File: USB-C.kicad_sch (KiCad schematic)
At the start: 32 parts, among them IC2 TPS2557QDRBTQ1, IC5 TPS2557QDRBTQ1, IC7 TPS2557QDRBTQ1, J10 USB_C_Receptacle, J5 USB_C_Receptacle_USB2.0_16P, J7 USB_C_Receptacle_USB2.0_16P

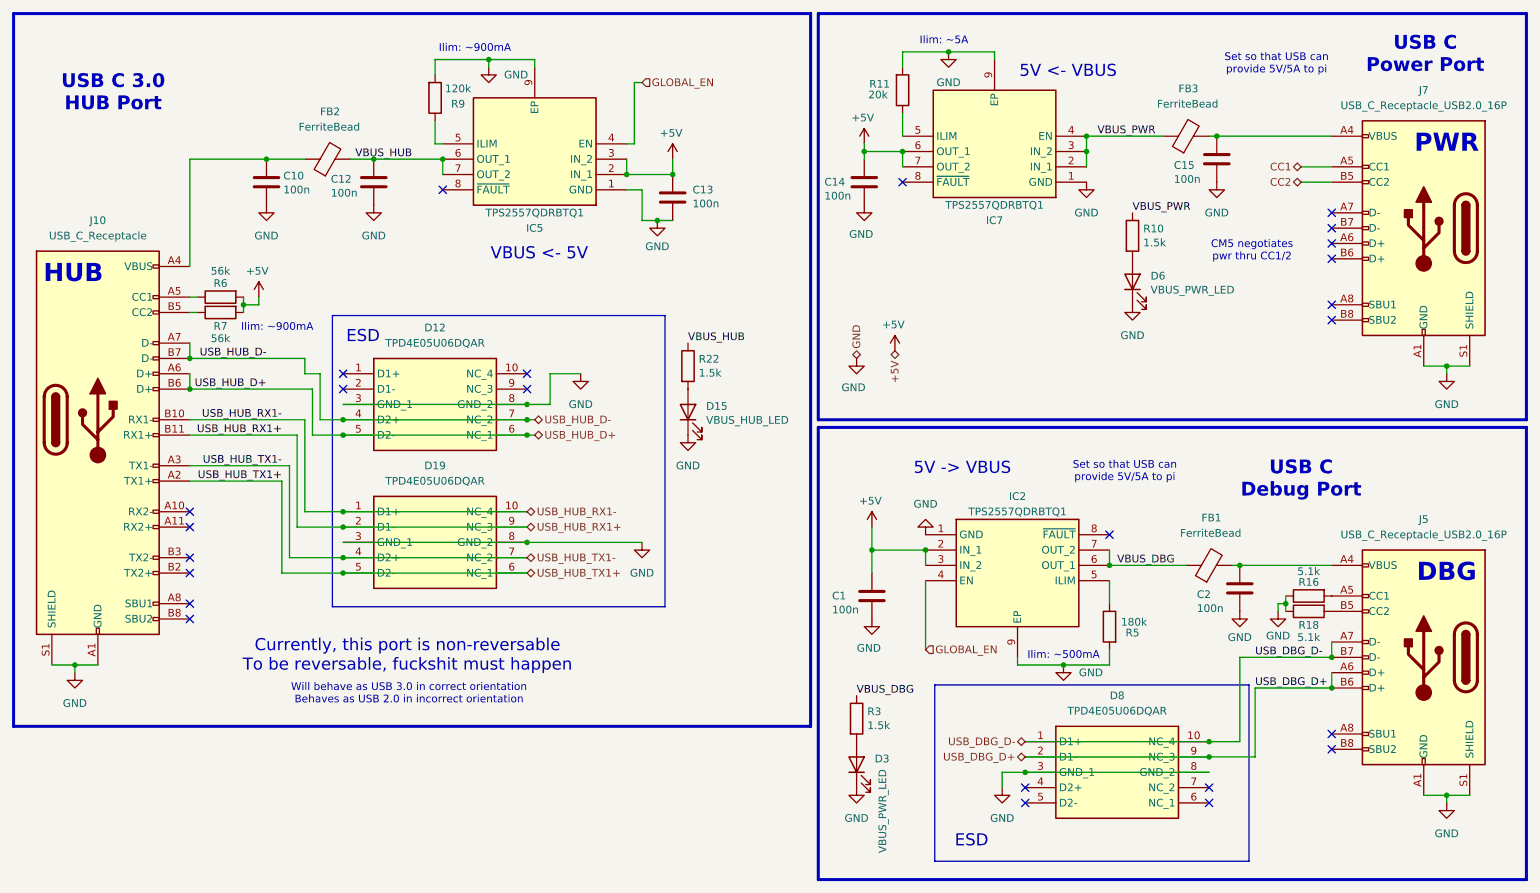
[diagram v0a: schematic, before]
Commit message: wow everything could not be worse
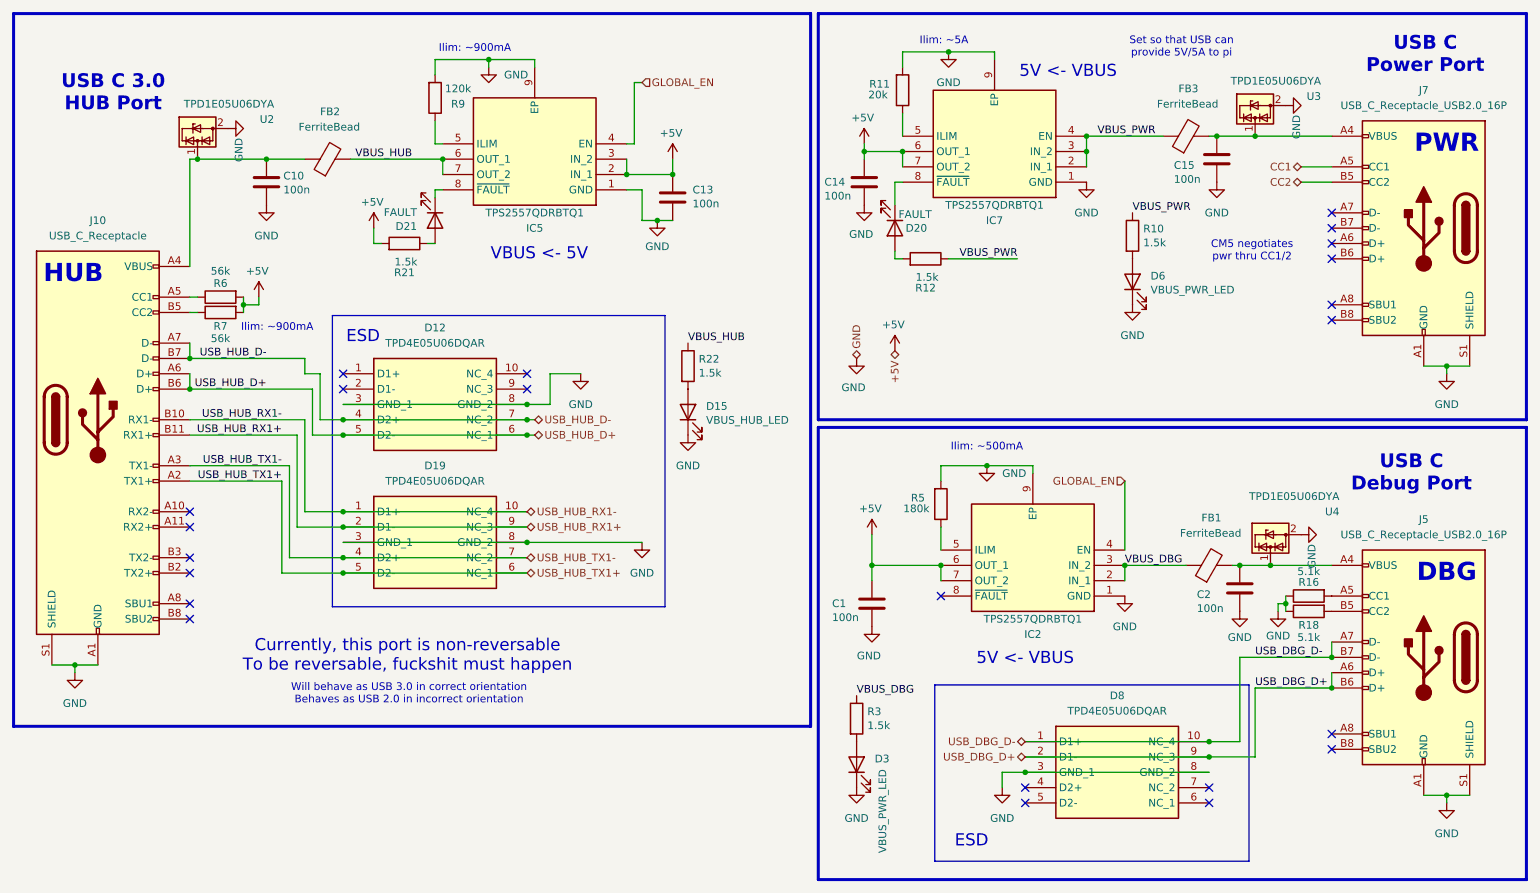
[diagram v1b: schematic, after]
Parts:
- removed C12: 100n, Capacitor_SMD:C_0603_1608Metric_Pad1.08x0.95mm_HandSolder, symbol Device:C
- added D20, D21: FAULT, LED_SMD:LED_0603_1608Metric_Pad1.05x0.95mm_HandSolder, symbol Device:LED
- added R12, R21: 1.5k, Resistor_SMD:R_0603_1608Metric_Pad0.98x0.95mm_HandSolder, symbol Device:R
- added U2, U3, U4: TPD1E05U06DYA, Diode_SMD:D_SOD-523, symbol Power_Protection:TPD1E05U06DYA
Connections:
- net +5V: now also IC2.6 (OUT_1), IC2.7 (OUT_2), R21.2; no longer IC2.2 (IN_1), IC2.3 (IN_2)
- net GND: now also U2.2 (GND), U3.2 (GND), U4.2 (GND)
- net VBUS_DBG: now also IC2.2 (IN_1), IC2.3 (IN_2); no longer IC2.6 (OUT_1), IC2.7 (OUT_2)
- net VBUS_PWR: now also R12.1
- net at C15.1, FB3.2, J7.A4 (VBUS)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: now also U3.1 (I/O)
- net at C10.1, FB2.1, J10.A4 (VBUS)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: now also U2.1 (I/O)
- net at C2.1, FB1.2, J5.A4 (VBUS)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: now also U4.1 (I/O)
- net at IC5.8 (~{FAULT}): now also D21.1 (K)
- net at IC7.8 (~{FAULT}): now also D20.1 (K)
- new net: D21.2 (A), R21.1
- new net: D20.2 (A), R12.2
- no-connect marks 25 -> 23
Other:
- note removed: "5V -> VBUS"
- moved on the sheet: C1, IC2, R5
